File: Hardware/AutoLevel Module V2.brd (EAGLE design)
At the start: 22.5 x 12.5 mm, 11 parts, among them X1 JST-XH-02-PIN-LONG-PAD, X2 JST-XH-02-PIN-LONG-PAD, X3 JST-XH-03-PIN-LONG-PAD

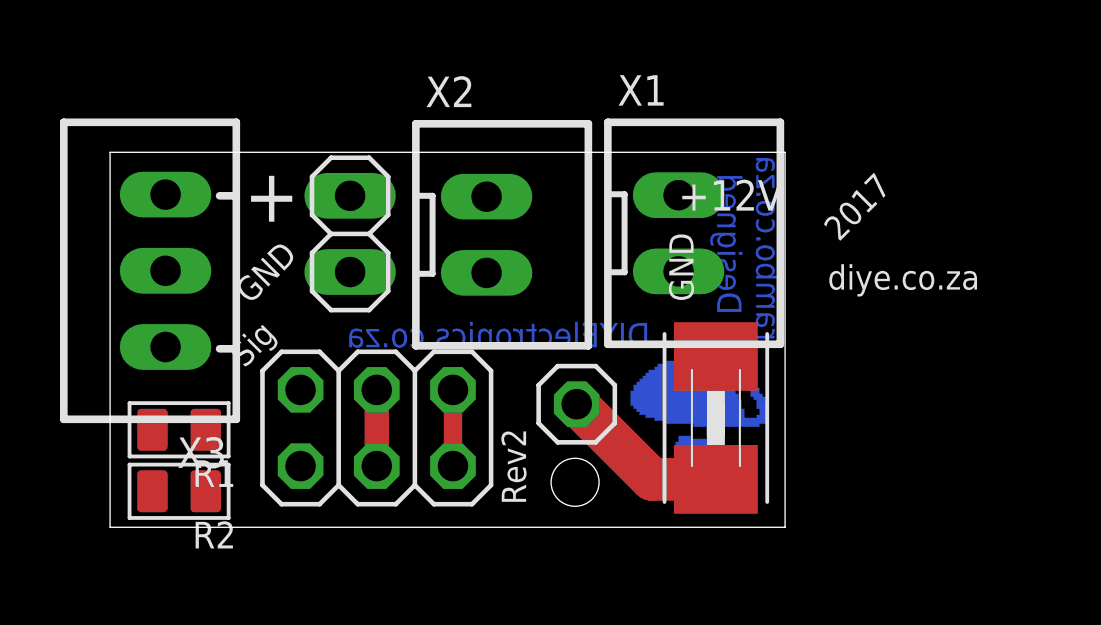
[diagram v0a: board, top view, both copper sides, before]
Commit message: RFM V2
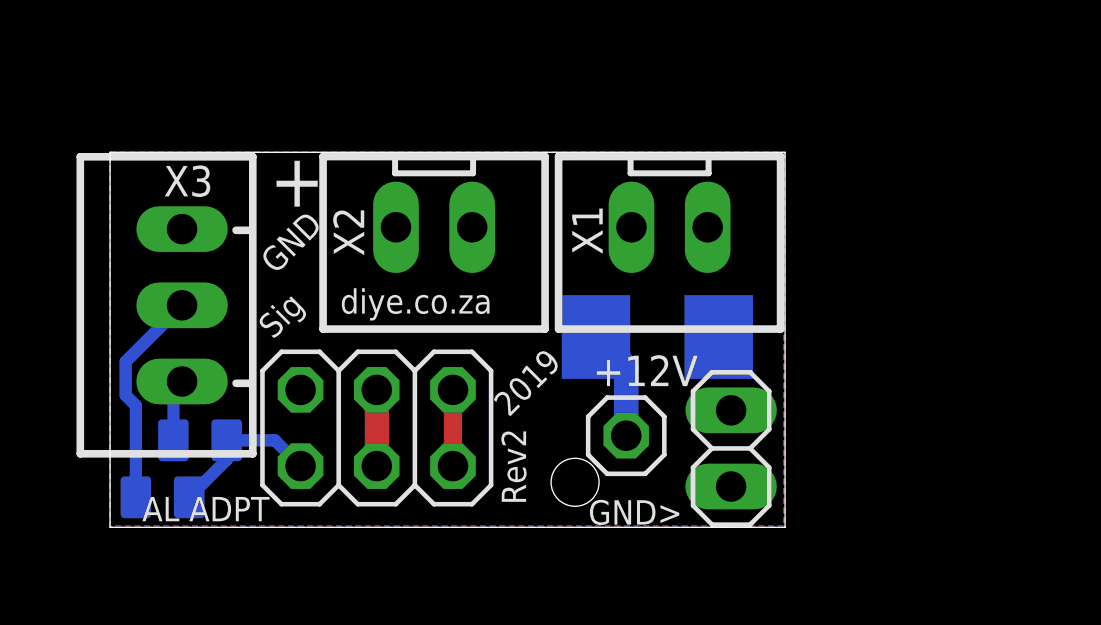
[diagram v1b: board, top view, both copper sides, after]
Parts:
- removed U$1: SHROOM5MM, RobThePyro:SHROOM
- moved U$2 17.4 mm to (8.60, 12.1), turned to 270 degrees
- moved JP2 14.6 mm to (20.7, 2.63)
- moved F1 3.33 mm to (18.2, 6.34), flipped to the bottom, turned to 180 degrees
- moved JP5 1.96 mm to (17.2, 3.05)
- moved X2 1.77 mm to (10.8, 10.0), turned to 180 degrees
- moved X3 1.27 mm to (2.40, 7.40)
- moved R1 0.78 mm to (3.00, 2.90), flipped to the bottom, turned to 90 degrees
- moved R2 0.59 mm to (1.75, 1.00), flipped to the bottom
- moved X1 0.36 mm to (18.6, 10.0), turned to 180 degrees
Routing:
- net GND: track 2.54 -> 9.86 mm
- net ZMIN: track 0.27 -> 5.23 mm
- net N$2: track 0.00 -> 2.08 mm
- net N$1: track 5.68 -> 3.71 mm
- added copper zone on layer 16, net +12V
- added copper zone on layer 1, net GND
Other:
- board text added: "2019"
- board text added: "DIYE.co.za"
- board text added: "GND>"
- board text added: "R1=15K R2=10K"
- board text removed: "2017"
- board text removed: "DIYElectronics.co.za"
